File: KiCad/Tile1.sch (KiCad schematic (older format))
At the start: 5 parts, among them J11 Conn_01x04, J12 Conn_01x08, J6 Conn_02x08_Odd_Even, U9 XUF216-512-FB236

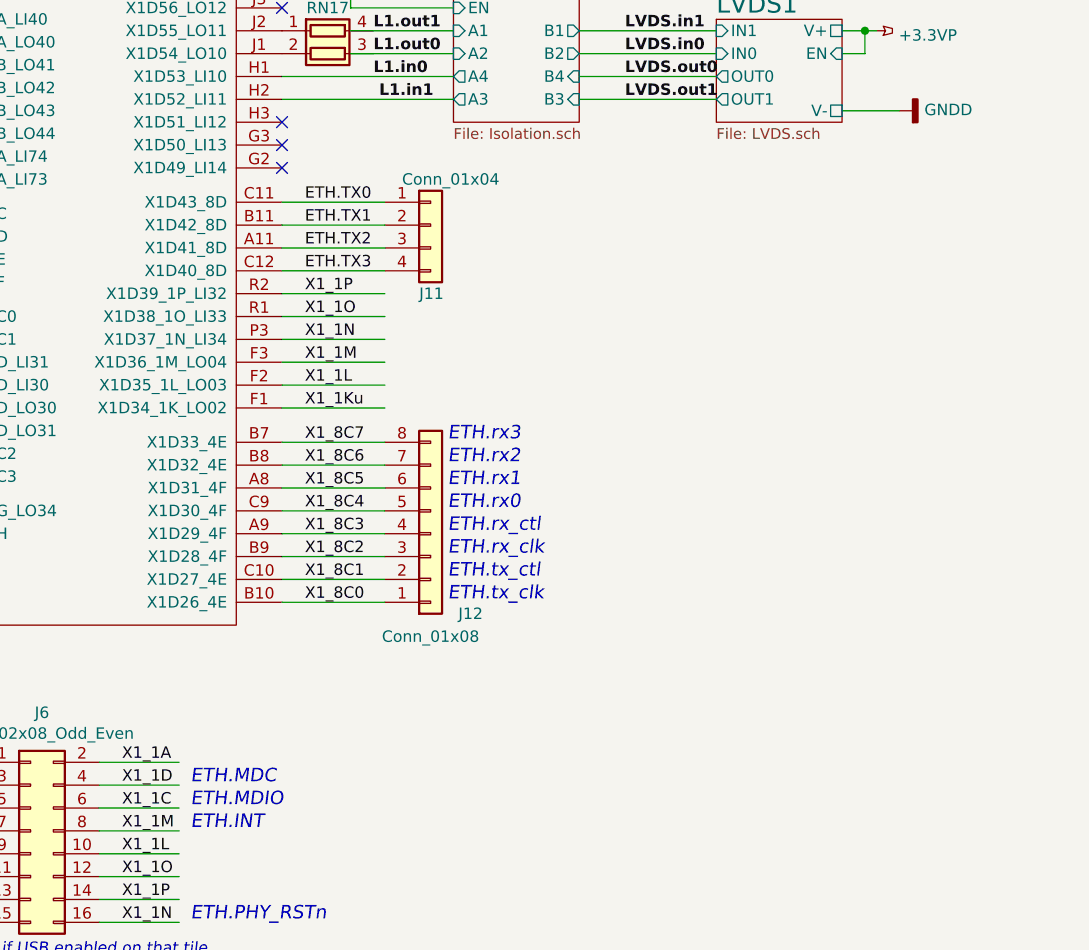
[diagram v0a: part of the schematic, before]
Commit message: Many small fixes
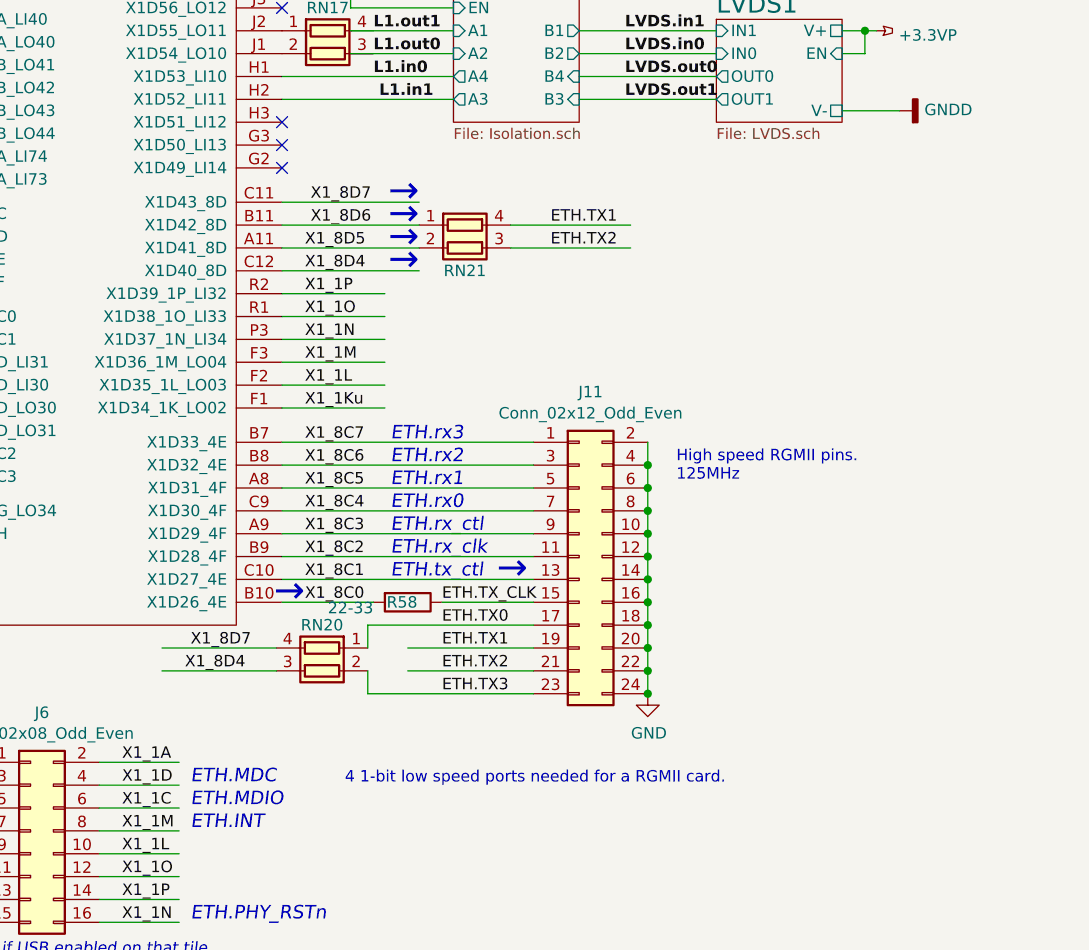
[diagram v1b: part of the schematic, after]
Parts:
- removed J11: Conn_01x04, Connector_PinSocket_2.54mm:PinSocket_1x04_P2.54mm_Vertical, symbol Connector_Generic:Conn_01x04
- removed J12: Conn_01x08, Connector_PinSocket_2.54mm:PinSocket_1x08_P2.54mm_Vertical, symbol Connector_Generic:Conn_01x08
- added J11: Conn_02x12_Odd_Even, Connector_PinSocket_2.54mm:PinSocket_2x12_P2.54mm_Vertical, symbol Connector_Generic:Conn_02x12_Odd_Even
- added R58: 22-33, Resistor_SMD:R_0603_1608Metric, symbol Device:R
- added RN20, RN21: 22-33R, Resistor_SMD:R_Array_Convex_2x0402, symbol Device:R_Pack02
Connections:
- net labels added: ETH.TX_CLK, X1_8D4, X1_8D5, X1_8D6, X1_8D7
- wire segments 82 -> 104
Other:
- note added: "4 1-bit low speed ports needed for a RGMII card."
- note added: "High speed RGMII pins.\n125MHz"
- note added: "→\n"
- note removed: "ETH.tx_clk\n"
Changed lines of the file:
@@
 Wire Wire Line
 	1650 3850 2350 3850
-Wire Wire Line
-	4150 4250 4600 4250
-Wire Wire Line
-	4150 4150 4600 4150
-Wire Wire Line
-	4150 4050 4600 4050
-Wire Wire Line
-	4150 3950 4600 3950
-Wire Wire Line
-	4150 3850 4600 3850
-Wire Wire Line
-	4150 3750 4600 3750
-Wire Wire Line
-	4150 3650 4600 3650
-Wire Wire Line
-	4150 3550 4600 3550
 Text Label 4250 4250 0    50   ~ 0
 X1_8C0
@@
 Wire Wire Line
 	2350 3700 1850 3700
-Wire Wire Line
-	4150 2500 4600 2500
-Wire Wire Line
-	4150 2600 4600 2600
-Wire Wire Line
-	4150 2700 4600 2700
-Wire Wire Line
-	4150 2800 4600 2800
 Wire Wire Line
 	2350 2400 1800 2400
@@
 Text Label 1950 3700 0    50   ~ 0
 X1D21
-Text Label 4250 2500 0    50   ~ 0
-ETH.TX0
 Text Label 4250 4150 0    50   ~ 0
 X1_8C1
@@
 NoConn ~ 1700 4050
 NoConn ~ 1800 2750
-$Comp
-L Connector_Generic:Conn_01x08 J?
-U 1 1 5CA7F8C7
-P 4800 3950
-AR Path="/5CA7F8C7" Ref="J?"  Part="1"
-AR Path="/5CA35A27/5CA7F8C7" Ref="J12"  Part="1"
-F 0 "J12" H 4975 4300 50  0000 C CNN
-F 1 "Conn_01x08" H 4800 4400 50  0000 C CNN
-F 2 "Connector_PinSocket_2.54mm:PinSocket_1x08_P2.54mm_Vertical" H 4800 3950 50  0001 C CNN
-F 3 "~" H 4800 3950 50  0001 C CNN
-F 4 "~" H 0   0   50  0001 C CNN "Part Number"
-	1    4800 3950
-	1    0    0    1
-$EndComp
 Wire Wire Line
 	4900 2050 4150 2050
@@
 NoConn ~ 1850 3600
 NoConn ~ 1850 3700
-Text Label 4250 2600 0    50   ~ 0
+Text Label 5325 2600 0    50   ~ 0
 ETH.TX1
-Text Label 4250 2700 0    50   ~ 0
+Text Label 5325 2700 0    50   ~ 0
 ETH.TX2
-Text Label 4250 2800 0    50   ~ 0
-ETH.TX3
-Text Notes 4875 3550 0    59   Italic 0
+Text Notes 4625 3550 0    59   Italic 0
 ETH.rx3
 Text Label 4550 1850 0    50   ~ 10
@@
 Text Label 4575 2050 0    50   ~ 10
 L1.in1
-$Comp
-L Connector_Generic:Conn_01x04 J?
-U 1 1 5CA7F92E
-P 4800 2600
-AR Path="/5CA7F92E" Ref="J?"  Part="1"
-AR Path="/5CA35A27/5CA7F92E" Ref="J11"  Part="1"
-F 0 "J11" H 4750 2300 50  0000 L CNN
-F 1 "Conn_01x04" H 4675 2800 50  0000 L CNN
-F 2 "Connector_PinSocket_2.54mm:PinSocket_1x04_P2.54mm_Vertical" H 4800 2600 50  0001 C CNN
-F 3 "~" H 4800 2600 50  0001 C CNN
-F 4 "~" H 0   0   50  0001 C CNN "Part Number"
-	1    4800 2600
-	1    0    0    -1
-$EndComp
 Wire Wire Line
 	1700 3200 2350 3200
@@
 Wire Wire Line
 	2350 1900 1750 1900
-Text Notes 4875 3650 0    59   Italic 0
+Text Notes 4625 3650 0    59   Italic 0
 ETH.rx2
-Text Notes 4875 3750 0    59   Italic 0
+Text Notes 4625 3750 0    59   Italic 0
 ETH.rx1
-Text Notes 4875 3850 0    59   Italic 0
+Text Notes 4625 3850 0    59   Italic 0
 ETH.rx0\n
-Text Notes 4875 3950 0    59   Italic 0
+Text Notes 4625 3950 0    59   Italic 0
 ETH.rx_ctl\n
-Text Notes 4875 4050 0    59   Italic 0
+Text Notes 4625 4050 0    59   Italic 0
 ETH.rx_clk\n
-Text Notes 4875 4150 0    59   Italic 0
+Text Notes 4625 4150 0    59   Italic 0
 ETH.tx_ctl\n
-Text Notes 4875 4250 0    59   Italic 0
-ETH.tx_clk\n
 $Comp
 L Device:R_Pack02 RN?
@@
 Wire Wire Line
 	4450 1850 4900 1850
+$Comp
+L Connector_Generic:Conn_02x12_Odd_Even J11
+U 1 1 5C357C1E
+P 5450 4050
+F 0 "J11" H 5500 4770 50  0000 C CNN
+F 1 "Conn_02x12_Odd_Even" H 5500 4677 50  0000 C CNN
+F 2 "Connector_PinSocket_2.54mm:PinSocket_2x12_P2.54mm_Vertical" H 5450 4050 50  0001 C CNN
+F 3 "~" H 5450 4050 50  0001 C CNN
+	1    5450 4050
+	1    0    0    -1
+$EndComp
+Wire Wire Line
+	4150 4250 4550 4250
+Wire Wire Line
+	4150 4150 5250 4150
+Wire Wire Line
+	4150 4050 5250 4050
+Wire Wire Line
+	4150 3950 5250 3950
+Wire Wire Line
+	4150 3850 5250 3850
+Wire Wire Line
+	4150 3750 5250 3750
+Wire Wire Line
+	4150 3650 5250 3650
+Wire Wire Line
+	4150 3550 5250 3550
+Wire Wire Line
+	4150 2500 4750 2500
+Wire Wire Line
+	4150 2600 4750 2600
+Wire Wire Line
+	4150 2700 4750 2700
+Wire Wire Line
+	4150 2800 4750 2800
+$Comp
+L power:GND #PWR?
+U 1 1 5C382B2B
+P 5750 4650
+AR Path="/5C382B2B" Ref="#PWR?"  Part="1"
+AR Path="/5CA35A27/5C382B2B" Ref="#PWR0117"  Part="1"
+F 0 "#PWR0117" H 5750 4400 50  0001 C CNN
+F 1 "GND" H 5755 4477 50  0000 C CNN
+F 2 "" H 5750 4650 50  0001 C CNN
+F 3 "" H 5750 4650 50  0001 C CNN
+	1    5750 4650
+	1    0    0    -1
+$EndComp
+Connection ~ 5750 3650
+Wire Wire Line
+	5750 3650 5750 3550
+Connection ~ 5750 3750
+Wire Wire Line
+	5750 3750 5750 3650
+Connection ~ 5750 3850
+Wire Wire Line
+	5750 3850 5750 3750
+Connection ~ 5750 3950
+Wire Wire Line
+	5750 3950 5750 3850
+Connection ~ 5750 4050
+Wire Wire Line
+	5750 4050 5750 3950
+Connection ~ 5750 4150
+Wire Wire Line
+	5750 4150 5750 4050
+Connection ~ 5750 4250
+Wire Wire Line
+	5750 4250 5750 4150
+Text Notes 4425 5050 0    50   ~ 0
+4 1-bit low speed ports needed for a RGMII card.
+Text Notes 5875 3725 0    50   ~ 0
+High speed RGMII pins.\n125MHz
+Wire Wire Line
+	5750 4250 5750 4350
+Connection ~ 5750 4350
+Wire Wire Line
+	5750 4350 5750 4450
+Connection ~ 5750 4450
+Wire Wire Line
+	5750 4450 5750 4550
+Connection ~ 5750 4550
+Wire Wire Line
+	5750 4550 5750 4650
+Wire Wire Line
+	5250 4450 4700 4450
+Wire Wire Line
+	5250 4550 4700 4550
+Text Label 4850 4350 0    50   ~ 0
+ETH.TX0
+Text Label 4850 4450 0    50   ~ 0
+ETH.TX1
+Text Label 4850 4550 0    50   ~ 0
+ETH.TX2
+Text Label 4850 4650 0    50   ~ 0
+ETH.TX3
+Connection ~ 5750 4650
+Text Notes 4750 2525 2    118  ~ 0
+→\n
+Text Notes 4750 2625 2    118  ~ 0
+→\n
+Text Notes 4750 2725 2    118  ~ 0
+→\n
+Text Notes 4750 2825 2    118  ~ 0
+→\n
+Text Notes 5225 4175 2    118  ~ 0
+→\n
+Text Notes 4250 4275 2    118  ~ 0
+→\n
+$Comp
+L Device:R_Pack02 RN?
+U 1 1 5C3CB19F
+P 4325 4550
+AR Path="/5C3CB19F" Ref="RN?"  Part="1"
+AR Path="/5CA35A27/5C3CB19F" Ref="RN20"  Part="1"
+F 0 "RN20" V 4125 4550 50  0000 C CNN
+F 1 "22-33R" V 4459 4550 50  0001 C CNN
+F 2 "Resistor_SMD:R_Array_Convex_2x0402" V 4500 4550 50  0001 C CNN
+F 3 "~" H 4325 4550 50  0001 C CNN
+F 4 "~" H -2900 1225 50  0001 C CNN "Part Number"
+	1    4325 4550
+	0    -1   1    0
+$EndComp
+Wire Wire Line
+	5150 2600 5675 2600
+$Comp
+L Device:R_Pack02 RN?
+U 1 1 5C3CB213
+P 4950 2700
+AR Path="/5C3CB213" Ref="RN?"  Part="1"
+AR Path="/5CA35A27/5C3CB213" Ref="RN21"  Part="1"
+F 0 "RN21" V 5050 2700 50  0000 C CNN
+F 1 "22-33R" V 5084 2700 50  0001 C CNN
+F 2 "Resistor_SMD:R_Array_Convex_2x0402" V 5125 2700 50  0001 C CNN
+F 3 "~" H 4950 2700 50  0001 C CNN
+F 4 "~" H -2275 -625 50  0001 C CNN "Part Number"
+	1    4950 2700
+	0    1    1    0
+$EndComp
+Wire Wire Line
+	5150 2700 5675 2700
+Wire Wire Line
+	4525 4450 4525 4350
+Wire Wire Line
+	4525 4350 5250 4350
+Wire Wire Line
+	4525 4650 4525 4550
+Wire Wire Line
+	4525 4650 5250 4650
+Wire Wire Line
+	3625 4550 4125 4550
+Wire Wire Line
+	4125 4450 3625 4450
+Text Label 4250 2800 0    50   ~ 0
+X1_8D4
+Text Label 4250 2700 0    50   ~ 0
+X1_8D5
+Text Label 4275 2600 0    50   ~ 0
+X1_8D6
+Text Label 4275 2500 0    50   ~ 0
+X1_8D7
+Text Label 3750 4450 0    50   ~ 0
+X1_8D7
+Text Label 3725 4550 0    50   ~ 0
+X1_8D4
+$Comp
+L Device:R R58
+U 1 1 5C3E9BF7
+P 4700 4250
+F 0 "R58" V 4700 4225 50  0000 C CNN
+F 1 "22-33" V 4725 4000 50  0000 C CNN
+F 2 "Resistor_SMD:R_0603_1608Metric" V 4630 4250 50  0001 C CNN
+F 3 "~" H 4700 4250 50  0001 C CNN
+	1    4700 4250
+	0    1    1    0
+$EndComp
+Wire Wire Line
+	4850 4250 5250 4250
+Text Label 4850 4250 0    50   ~ 0
+ETH.TX_CLK
 $EndSCHEMATC
